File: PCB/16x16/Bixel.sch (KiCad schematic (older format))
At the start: 261 parts, among them J1 Conn_01x22, J2 Screw_Terminal_01x02, U1 74HC595, U2 74HC595

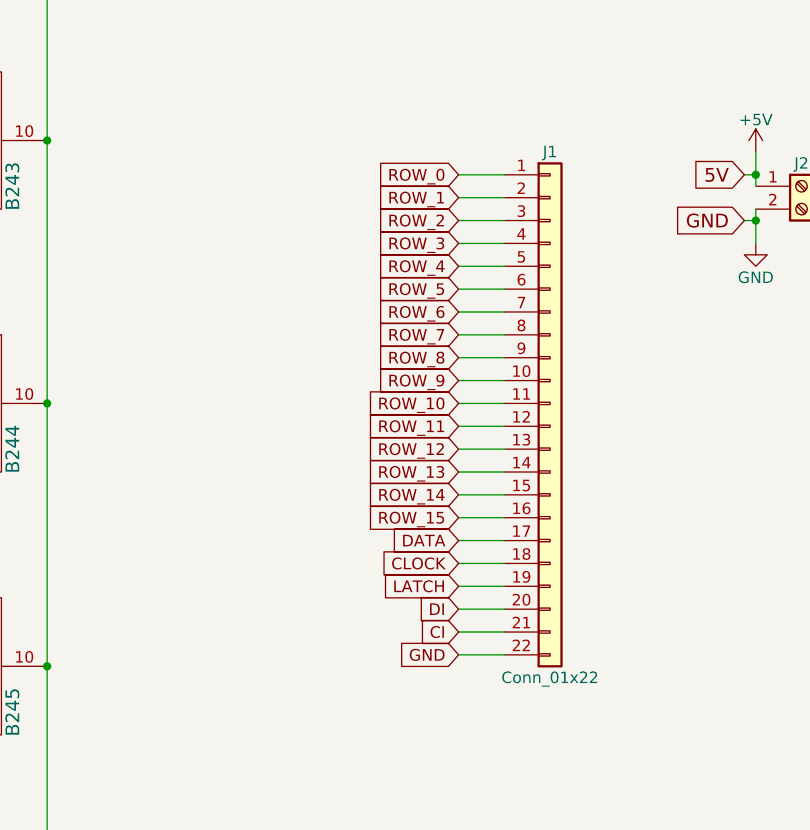
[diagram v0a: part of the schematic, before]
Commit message: More work on PCB layout
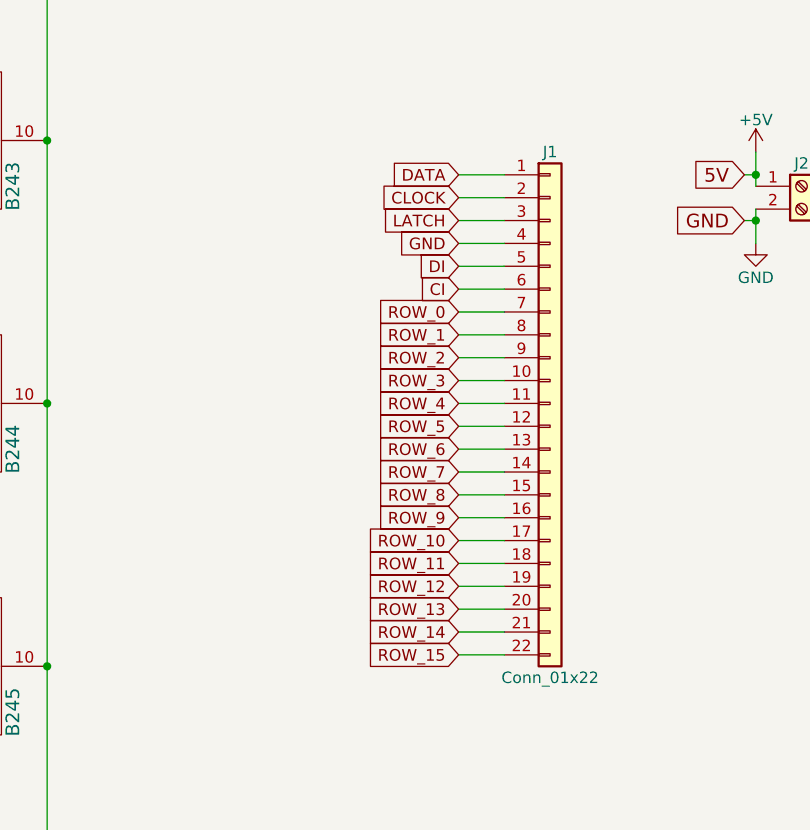
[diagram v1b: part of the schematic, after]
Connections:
- net CI: now also J1.6 (Pin_6); no longer J1.21 (Pin_21)
- net CLOCK: now also J1.2 (Pin_2); no longer J1.18 (Pin_18)
- net DATA: now also J1.1 (Pin_1); no longer J1.17 (Pin_17)
- net DI: now also J1.5 (Pin_5); no longer J1.20 (Pin_20)
- net GND: now also J1.4 (Pin_4); no longer J1.22 (Pin_22)
- net LATCH: now also J1.3 (Pin_3); no longer J1.19 (Pin_19)
- net ROW_0: now also J1.7 (Pin_7); no longer J1.1 (Pin_1)
- net ROW_1: now also J1.8 (Pin_8); no longer J1.2 (Pin_2)
- net ROW_10: now also J1.17 (Pin_17); no longer J1.11 (Pin_11)
- net ROW_11: now also J1.18 (Pin_18); no longer J1.12 (Pin_12)
- net ROW_12: now also J1.19 (Pin_19); no longer J1.13 (Pin_13)
- net ROW_13: now also J1.20 (Pin_20); no longer J1.14 (Pin_14)
- net ROW_14: now also J1.21 (Pin_21); no longer J1.15 (Pin_15)
- net ROW_15: now also J1.22 (Pin_22); no longer J1.16 (Pin_16)
- net ROW_2: now also J1.9 (Pin_9); no longer J1.3 (Pin_3)
- net ROW_3: now also J1.10 (Pin_10); no longer J1.4 (Pin_4)
- net ROW_4: now also J1.11 (Pin_11); no longer J1.5 (Pin_5)
- net ROW_5: now also J1.12 (Pin_12); no longer J1.6 (Pin_6)
- net ROW_6: now also J1.13 (Pin_13); no longer J1.7 (Pin_7)
- net ROW_7: now also J1.14 (Pin_14); no longer J1.8 (Pin_8)
- net ROW_8: now also J1.15 (Pin_15); no longer J1.9 (Pin_9)
- net ROW_9: now also J1.16 (Pin_16); no longer J1.10 (Pin_10)
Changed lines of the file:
@@
 Wire Wire Line
 	26050 4150 26150 4150
+Text GLabel 24400 6000 0    51   Input ~ 0
+ROW_0
+Text GLabel 24400 6100 0    51   Input ~ 0
+ROW_1
+Text GLabel 24400 6200 0    51   Input ~ 0
+ROW_2
+Text GLabel 24400 6300 0    51   Input ~ 0
+ROW_3
+Text GLabel 24400 6400 0    51   Input ~ 0
+ROW_4
+Text GLabel 24400 6500 0    51   Input ~ 0
+ROW_5
+Text GLabel 24400 6600 0    51   Input ~ 0
+ROW_6
+Text GLabel 24400 6700 0    51   Input ~ 0
+ROW_7
+Text GLabel 24400 6800 0    51   Input ~ 0
+ROW_8
+Text GLabel 24400 6900 0    51   Input ~ 0
+ROW_9
+Text GLabel 24400 7000 0    51   Input ~ 0
+ROW_10
+Text GLabel 24400 7100 0    51   Input ~ 0
+ROW_11
+Text GLabel 24400 7200 0    51   Input ~ 0
+ROW_12
+Text GLabel 24400 7300 0    51   Input ~ 0
+ROW_13
+Text GLabel 24400 7400 0    51   Input ~ 0
+ROW_14
+Text GLabel 24400 7500 0    51   Input ~ 0
+ROW_15
 Text GLabel 24400 5400 0    51   Input ~ 0
-ROW_0
+DATA
 Text GLabel 24400 5500 0    51   Input ~ 0
-ROW_1
+CLOCK
 Text GLabel 24400 5600 0    51   Input ~ 0
-ROW_2
+LATCH
 Text GLabel 24400 5700 0    51   Input ~ 0
-ROW_3
-Text GLabel 24400 5800 0    51   Input ~ 0
-ROW_4
-Text GLabel 24400 5900 0    51   Input ~ 0
-ROW_5
-Text GLabel 24400 6000 0    51   Input ~ 0
-ROW_6
-Text GLabel 24400 6100 0    51   Input ~ 0
-ROW_7
-Text GLabel 24400 6200 0    51   Input ~ 0
-ROW_8
-Text GLabel 24400 6300 0    51   Input ~ 0
-ROW_9
-Text GLabel 24400 6400 0    51   Input ~ 0
-ROW_10
-Text GLabel 24400 6500 0    51   Input ~ 0
-ROW_11
-Text GLabel 24400 6600 0    51   Input ~ 0
-ROW_12
-Text GLabel 24400 6700 0    51   Input ~ 0
-ROW_13
-Text GLabel 24400 6800 0    51   Input ~ 0
-ROW_14
-Text GLabel 24400 6900 0    51   Input ~ 0
-ROW_15
-Text GLabel 24400 7000 0    51   Input ~ 0
-DATA
-Text GLabel 24400 7100 0    51   Input ~ 0
-CLOCK
-Text GLabel 24400 7200 0    51   Input ~ 0
-LATCH
-Text GLabel 24400 7500 0    51   Input ~ 0
 GND
 $Comp
@@
 	1    0    0    -1
 $EndComp
-Text GLabel 24400 7300 0    51   Input ~ 0
+Text GLabel 24400 5800 0    51   Input ~ 0
 DI
-Text GLabel 24400 7400 0    51   Input ~ 0
+Text GLabel 24400 5900 0    51   Input ~ 0
 CI
 Text GLabel 8000 2350 1    51   Input ~ 0
